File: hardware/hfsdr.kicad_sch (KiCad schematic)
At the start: 52 parts, among them J1 USB_C_Receptacle_USB2.0_16P, SW1 RST, SW2 BOOT0, SW4 EC12E2430803, U3 CH32V30xRxTx

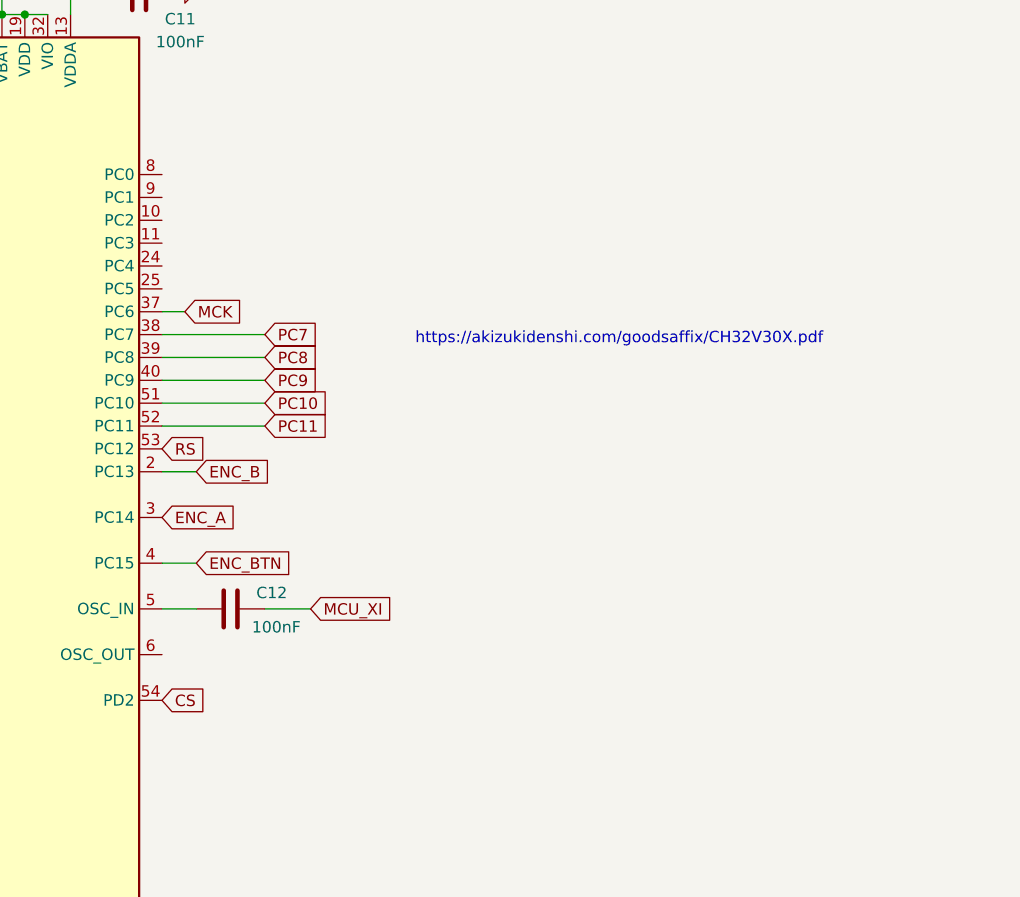
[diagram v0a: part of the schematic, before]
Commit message: feat: add front LEDs
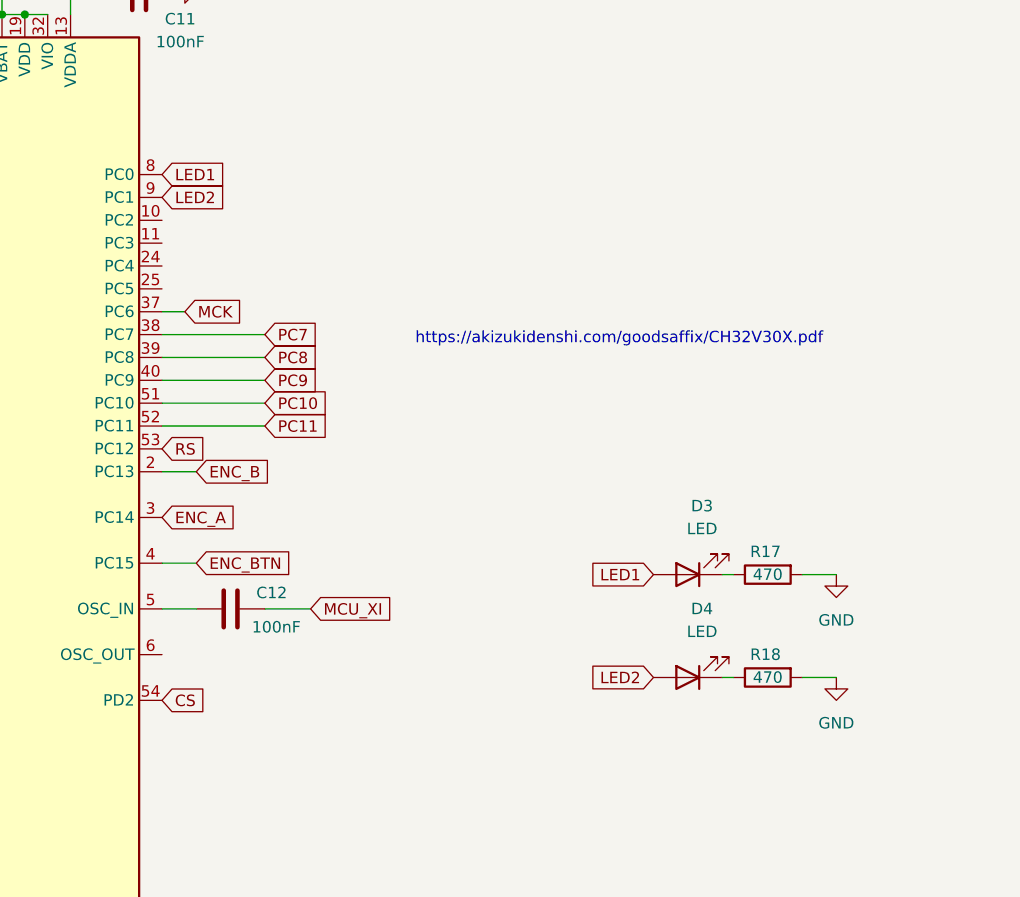
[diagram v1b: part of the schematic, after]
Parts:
- added D3, D4: LED, LED_SMD:LED_0603_1608Metric_Pad1.05x0.95mm_HandSolder, symbol Device:LED
- added R17, R18: 470, Resistor_SMD:R_0603_1608Metric_Pad0.98x0.95mm_HandSolder, symbol Device:R
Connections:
- net GND: now also R17.2, R18.2
- net LED1: now reaches U3.8 (PC0)
- net LED1: now also D3.2 (A)
- net LED2: now reaches U3.9 (PC1)
- net LED2: now also D4.2 (A)
- new net: D3.1 (K), R17.1
- new net: D4.1 (K), R18.1

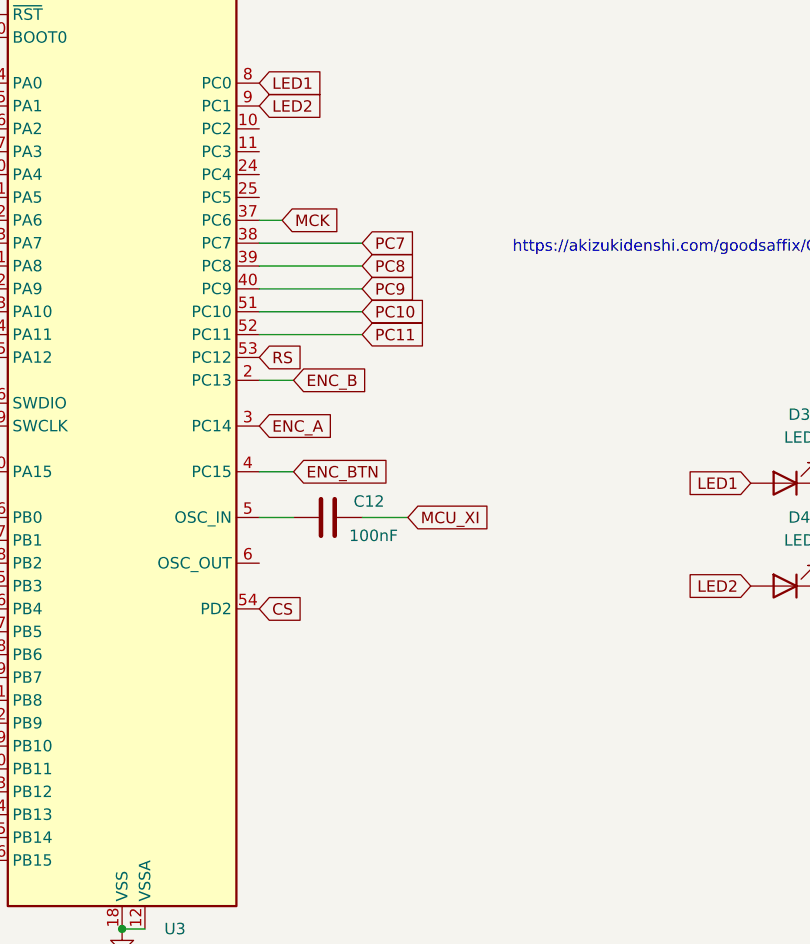
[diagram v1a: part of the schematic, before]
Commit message: Production ready
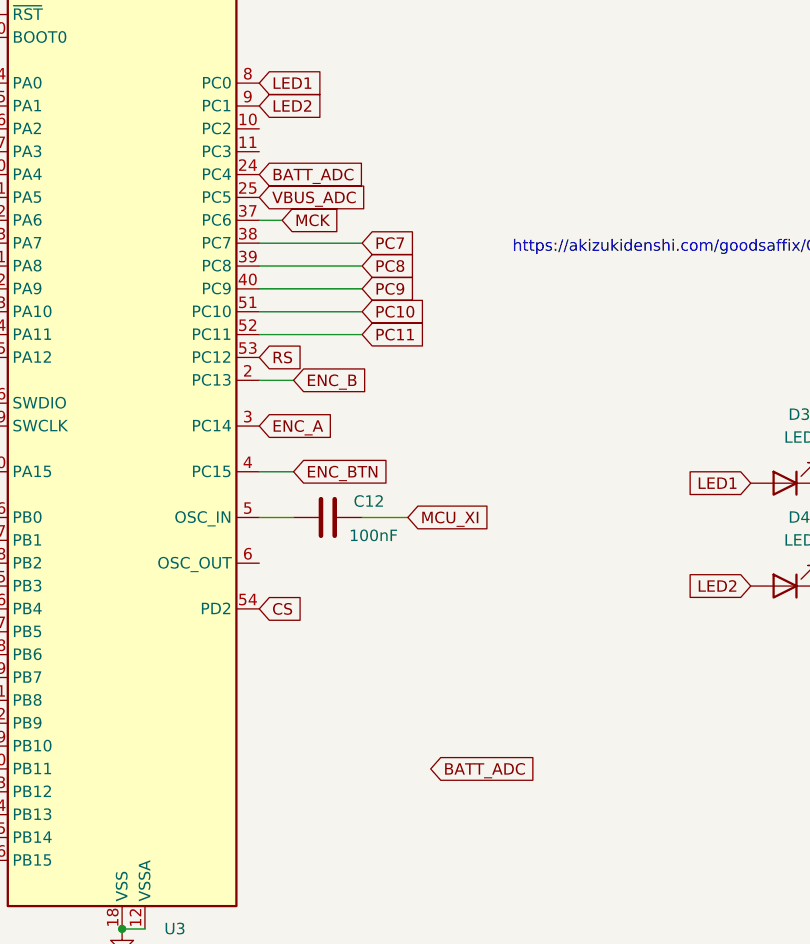
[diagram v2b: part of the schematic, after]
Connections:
- net BATT_ADC: now reaches U3.24 (PC4)
- net VBUS_ADC: now reaches U3.25 (PC5)
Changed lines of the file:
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@@
+		)
+	)
+	(global_label "BATT_ADC"
+		(shape input)
+		(at 168.91 77.47 0)
+		(fields_autoplaced yes)
+		(effects
+			(font
+				(size 1.27 1.27)
+			)
+			(justify left)
+		)
+		(property "Intersheetrefs" "${INTERSHEET_REFS}"
+			(at 180.7852 77.47 0)
+			(effects
+				(font
+					(size 1.27 1.27)
+				)
+				(justify left)
+				(hide yes)
+			)
 		)
 	)
@@
 		)
 	)
+	(global_label "BATT_ADC"
+		(shape input)
+		(at 187.96 143.51 0)
+		(fields_autoplaced yes)
+		(effects
+			(font
+				(size 1.27 1.27)
+			)
+			(justify left)
+		)
+		(property "Intersheetrefs" "${INTERSHEET_REFS}"
+			(at 199.8352 143.51 0)
+			(effects
+				(font
+					(size 1.27 1.27)
+				)
+				(justify left)
+				(hide yes)
+			)
+		)
+	)
 	(global_label "LED1"
 		(shape input)
@@
 				(hide yes)
 			)
+		)
+	)
+	(global_label "VBUS_ADC"
+		(shape input)
+		(at 168.91 80.01 0)
+		(fields_autoplaced yes)
+		(effects
+			(font
+				(size 1.27 1.27)
+			)
+			(justify left)
+		)
+		(property "Intersheetrefs" "${INTERSHEET_REFS}"
+			(at 181.39 80.01 0)
+			(effects
+				(font
+					(size 1.27 1.27)
+				)
+				(justify left)
+				(hide yes)
+			)
